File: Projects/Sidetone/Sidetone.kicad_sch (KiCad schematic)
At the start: 54 parts, among them Q1 2N3904, Q2 2N3904, Q3 2N3904, SW1 morse key, SW2 On/off, U1 4N35, U2 LM324, U3 LM386

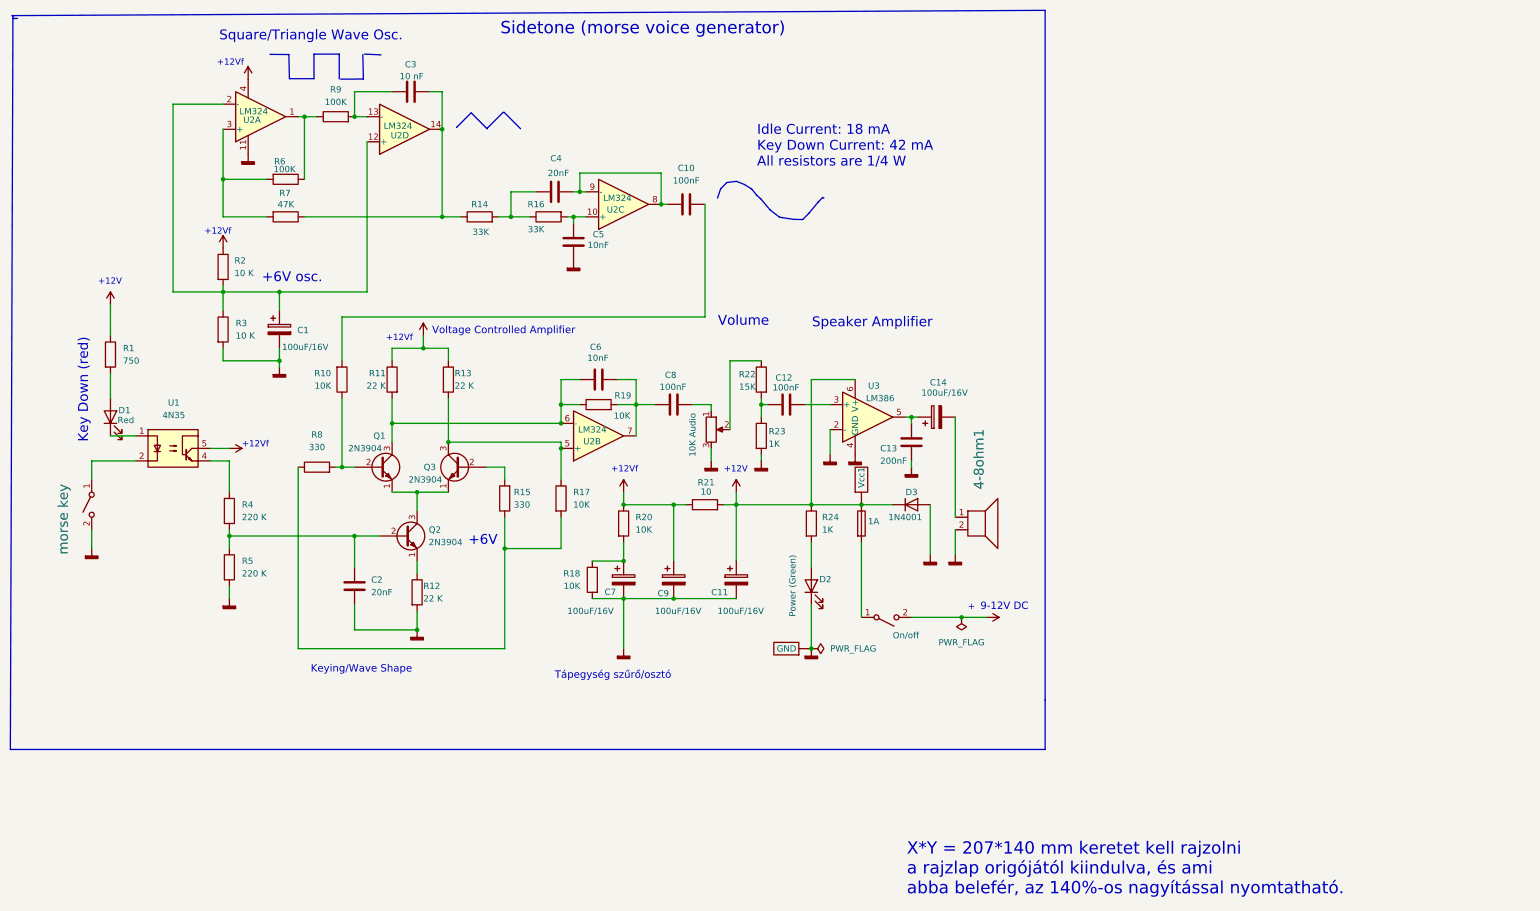
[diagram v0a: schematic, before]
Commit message: building pcb 20240222
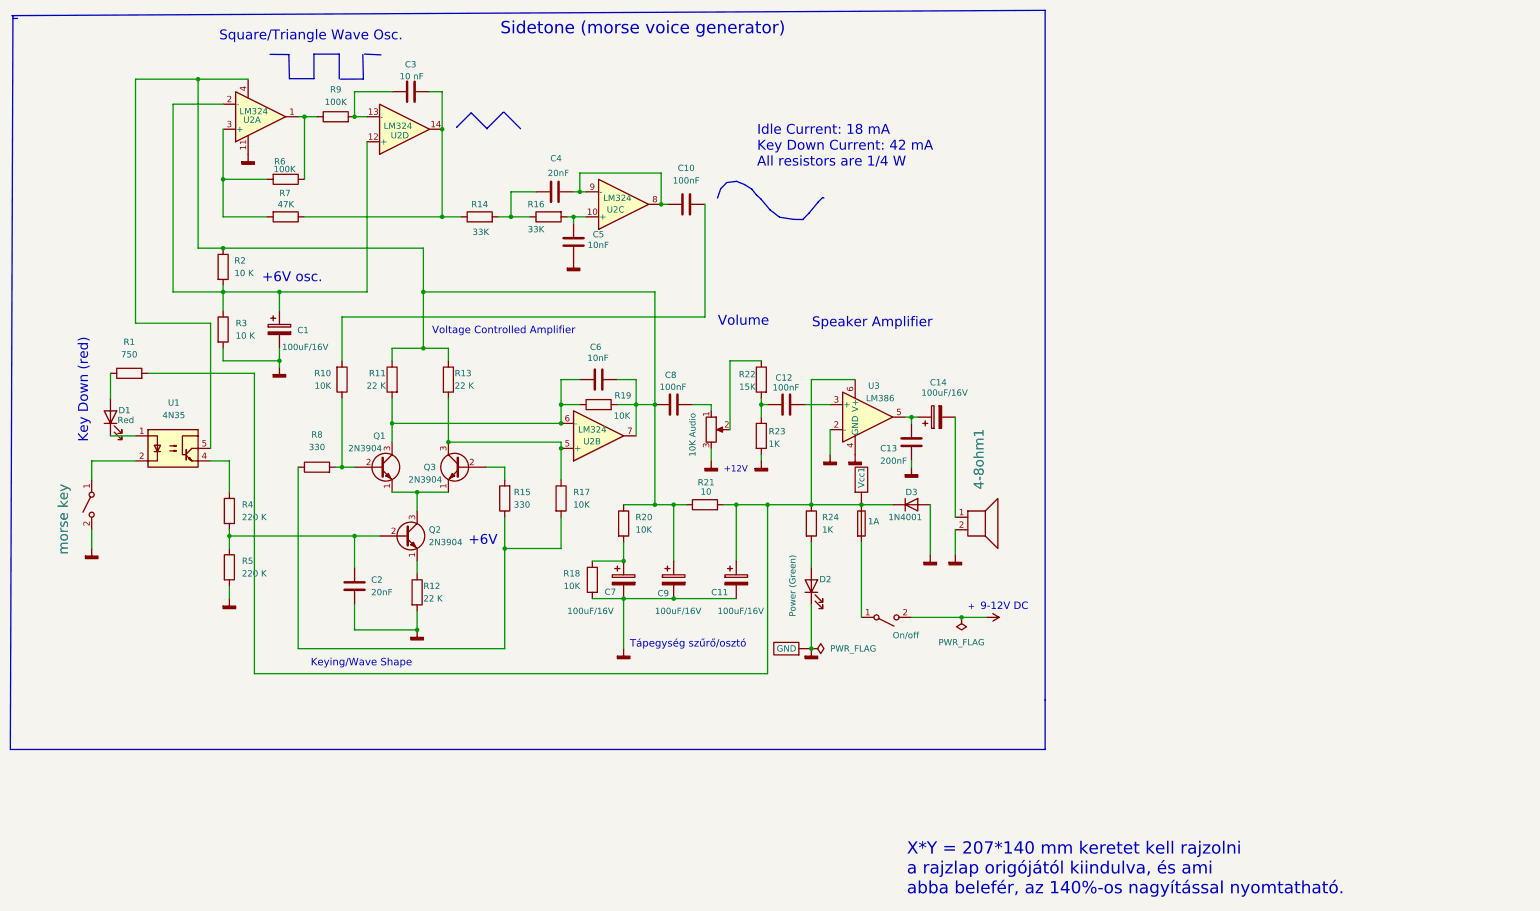
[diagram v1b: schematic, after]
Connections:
- net VCC: no longer C11.1, C9.1, D3.1 (K), F1.1, R1.1, R11.1, R13.1, R2.1, R20.1, R21.1, R21.2, R24.1, U1.5, U2.4 (V+), U3.6 (V+), Vcc1.
- net at C6.2, C8.1, R19.2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: now also C9.1, R11.1, R13.1, R2.1, R20.1, R21.1, U1.5, U2.4 (V+)
- net at R1.2: now also C11.1, D3.1 (K), F1.1, R21.2, R24.1, U3.6 (V+), Vcc1.; no longer D1.2 (A)
- new net: D1.2 (A), R1.1
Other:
- note removed: "+12Vf"
- moved on the sheet: R1
